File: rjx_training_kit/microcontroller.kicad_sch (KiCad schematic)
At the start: 25 parts, among them SW2 SW_Push, U1 STM32F407VGTx, Y1 8MHz, Y2 32.768kHz

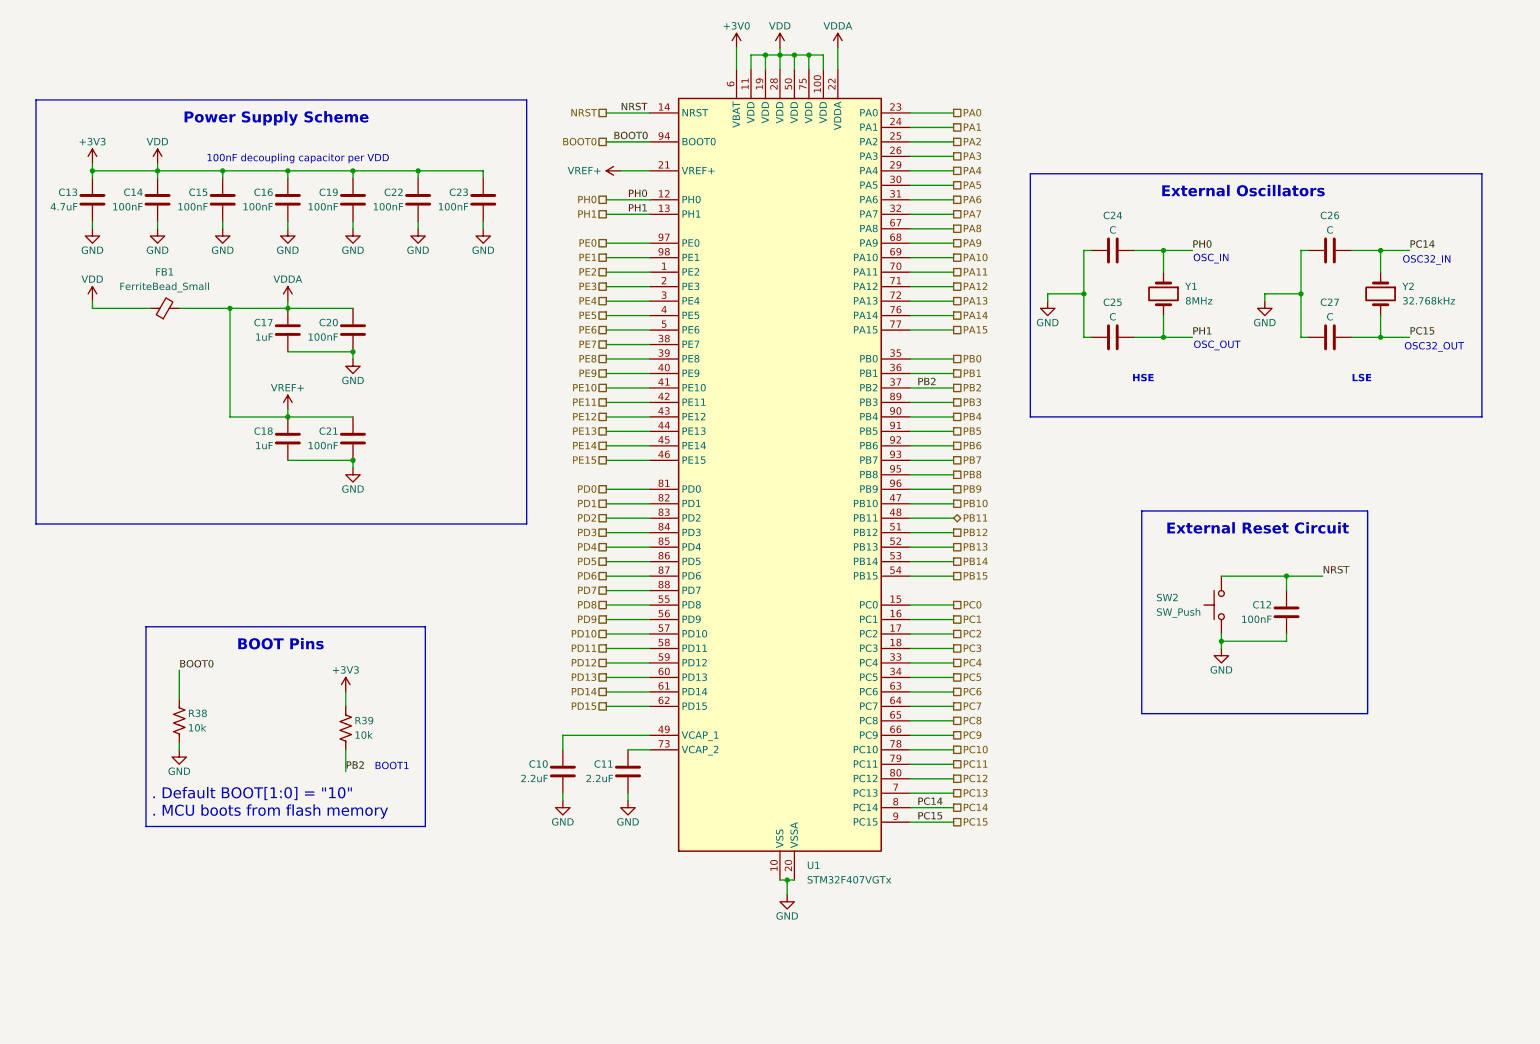
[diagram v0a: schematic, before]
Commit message: Update
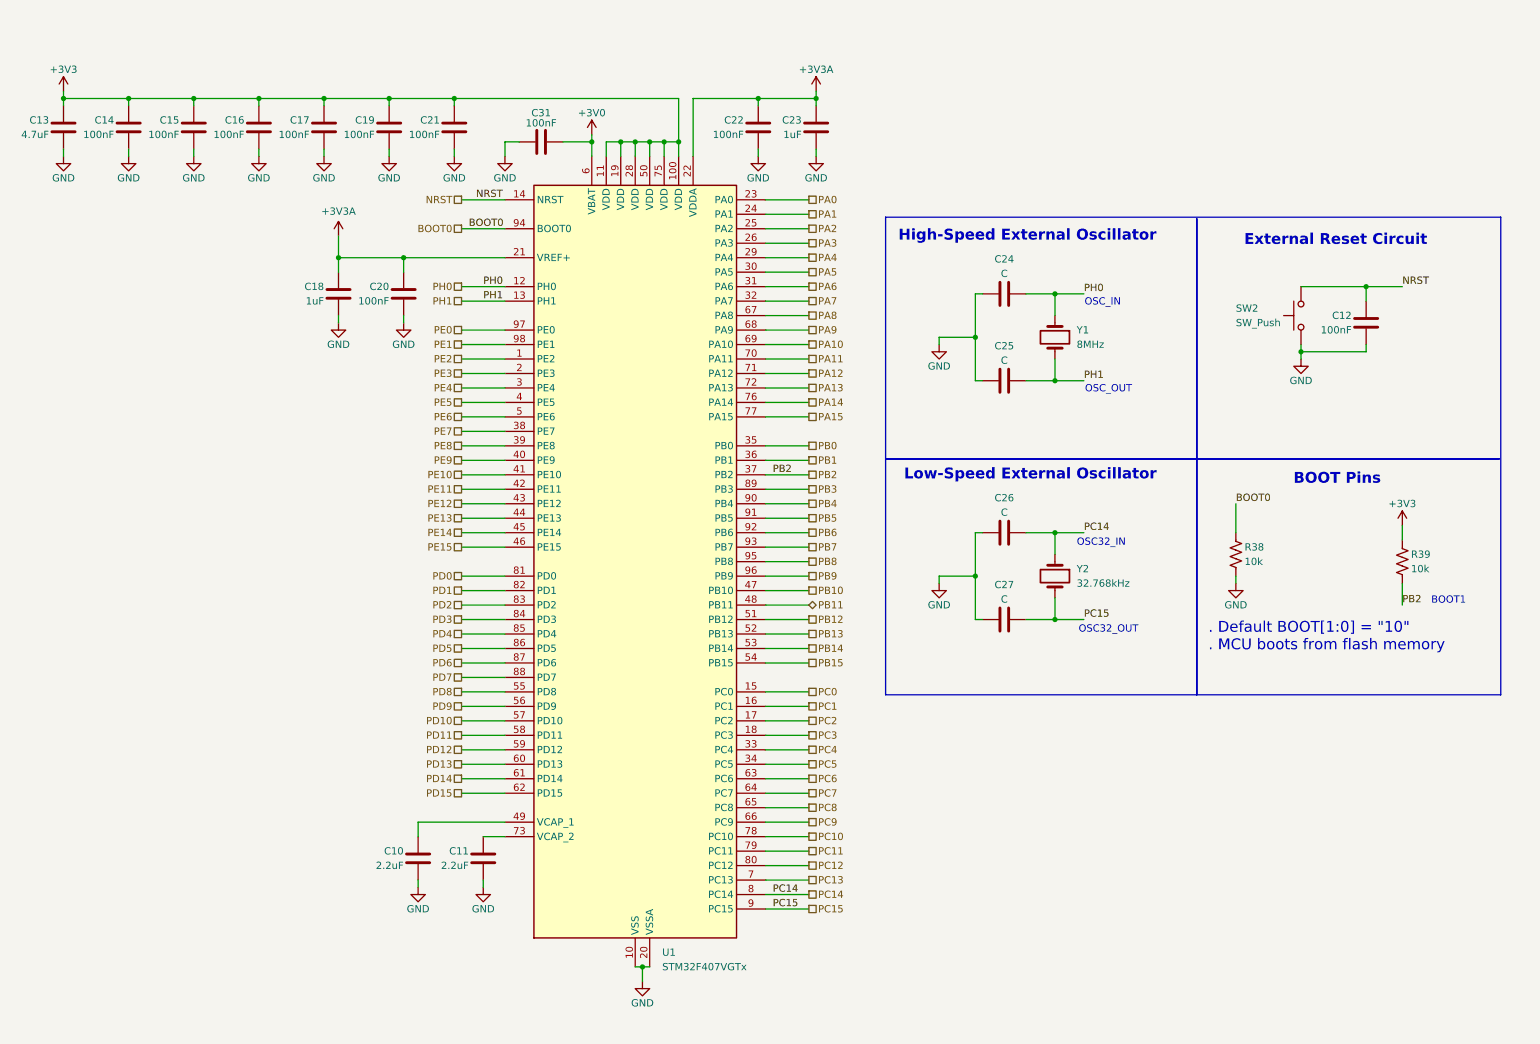
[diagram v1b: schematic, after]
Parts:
- removed FB1: FerriteBead_Small, symbol Device:FerriteBead_Small
- added C31: 100nF, symbol Device:C
- C17: value 1uF -> 100nF
- C23: value 100nF -> 1uF
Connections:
- net +3V0: now also C31.1
- net +3V3: now also C17.1, C21.1; no longer C22.1, C23.1
- net GND: now also C31.2
- net VDDA renamed +3V3A
- net +3V3A: now also C22.1, C23.1; no longer C17.1, C21.1
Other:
- note added: "High-Speed External Oscillator"
- note added: "Low-Speed External Oscillator"
- note removed: "100nF decoupling capacitor per VDD"
- note removed: "External Oscillators"
- note removed: "HSE"
- note removed: "LSE"
- note removed: "Power Supply Scheme"
- moved on the sheet: C10, C11, C12, C24, C25, C26, C27, R38, R39, SW2, U1, Y1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

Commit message: Update
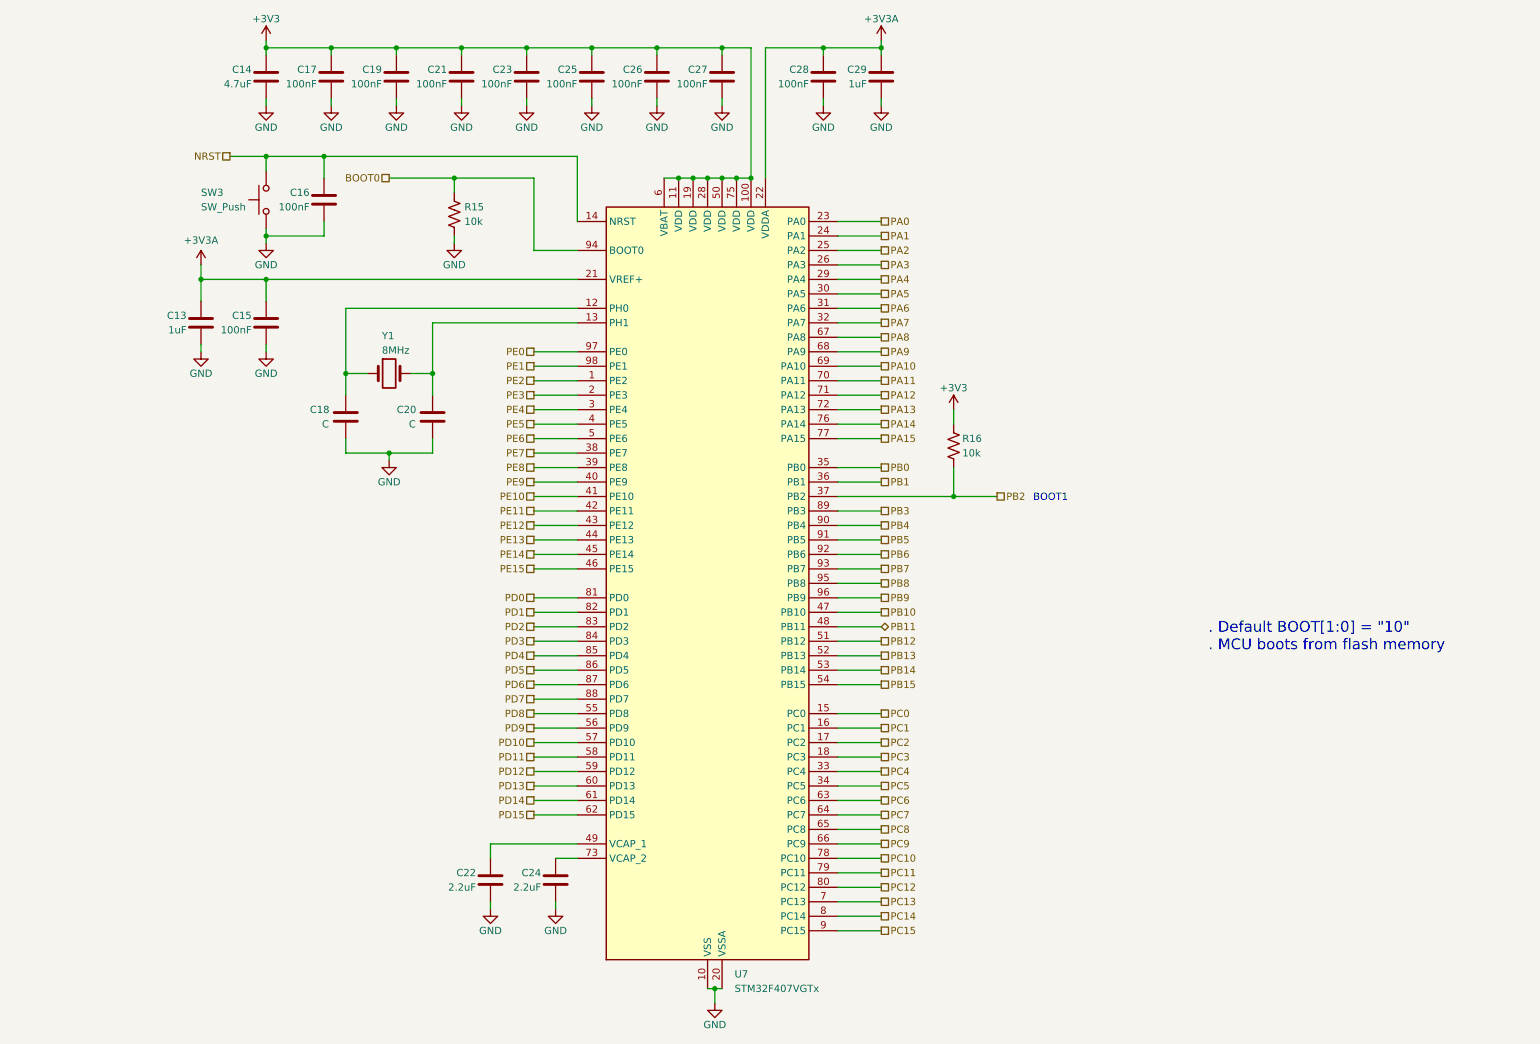
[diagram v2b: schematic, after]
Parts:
- removed C12, C31: 100nF, symbol Device:C
- removed C24, C25, C26: C, symbol Device:C
- removed R38: 10k, symbol Device:R_US
- removed SW2: SW_Push, symbol Switch:SW_Push
- removed Y2: 32.768kHz, symbol Device:Crystal
- added C16: 100nF, symbol Device:C
- added C18, C20: C, symbol Device:C
- added R15: 10k, symbol Device:R_US
- added SW3: SW_Push, symbol Switch:SW_Push
- C27: value C -> 100nF
- renumbered C18 to C13, C13 to C14, C20 to C15, C14 to C17, C15 to C19, C16 to C21, C10 to C22, C17 to C23, C11 to C24, C19 to C25, C21 to C26, C22 to C28, C23 to C29, R39 to R16, U1 to U7
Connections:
- net +3V0 is gone; now on net +3V3: U7.6 (VBAT)
- net +3V3: now also C27.1
- net BOOT0: now also R15.1
- net GND: now also C27.2, C16.2, C18.1, C20.1, R15.2, SW3.1; no longer C27.1
- net NRST: now also C16.1, SW3.2
- net PC15: no longer C27.2
- net PH0: no longer names the net of U7.12 (PH0), Y1.1
- net PH0: now also C18.2
- net PH1: no longer names the net of U7.13 (PH1), Y1.2
- net PH1: now also C20.2
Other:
- note removed: "BOOT Pins"
- note removed: "External Reset Circuit"
- note removed: "High-Speed External Oscillator"
- note removed: "Low-Speed External Oscillator"
- note removed: "OSC32_IN"
- note removed: "OSC32_OUT"
- note removed: "OSC_IN"
- note removed: "OSC_OUT"
- moved on the sheet: C13, C14, C15, C17, C19, C21, C22, C23, C24, C25, C26, C28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
